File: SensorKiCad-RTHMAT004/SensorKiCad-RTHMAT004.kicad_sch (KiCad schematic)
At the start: 19 parts, among them J1 Conn_02x14_Odd_Even, Q1 SS8050

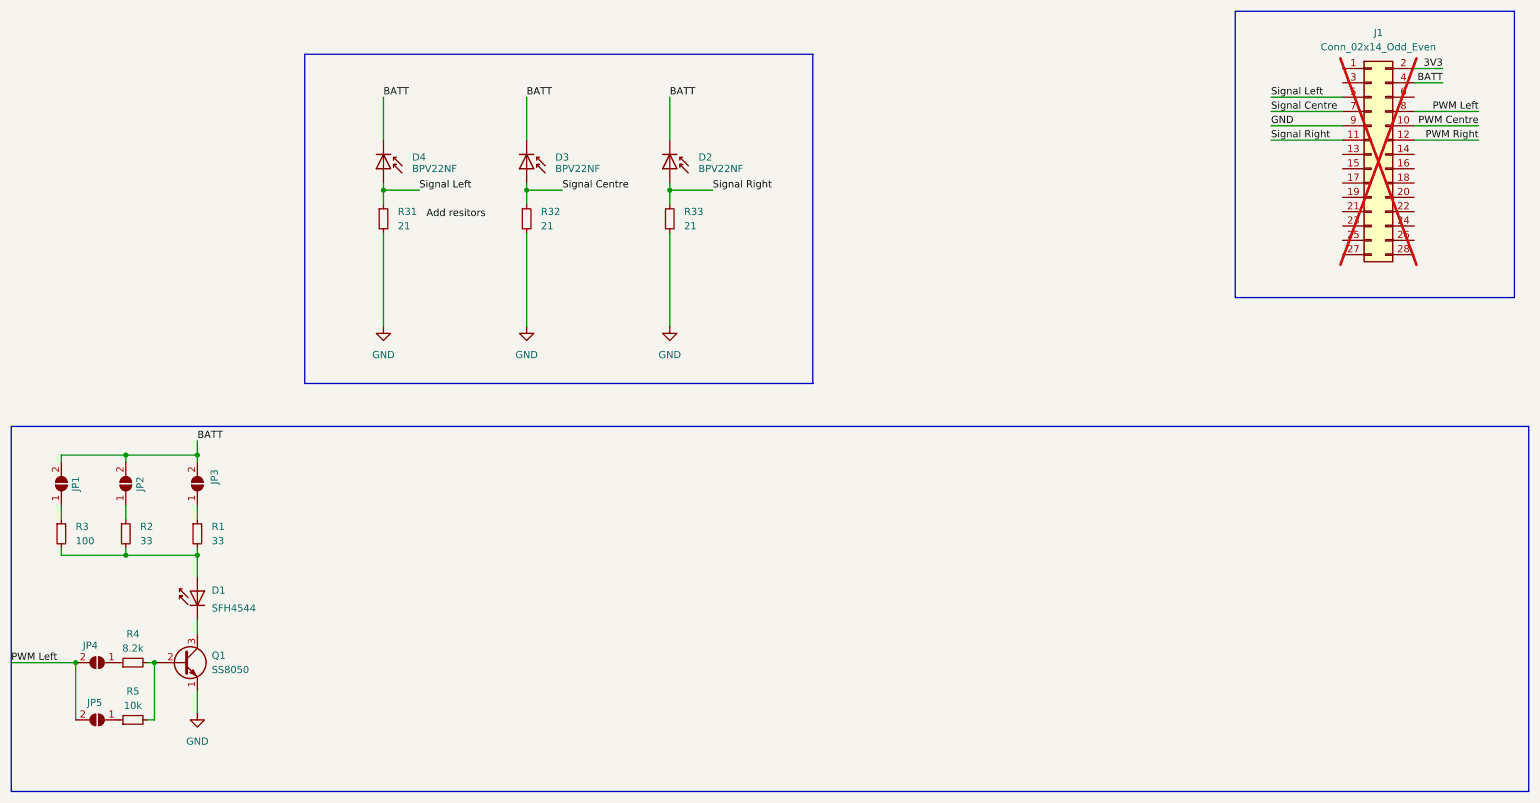
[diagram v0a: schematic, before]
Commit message: Finalising PCB
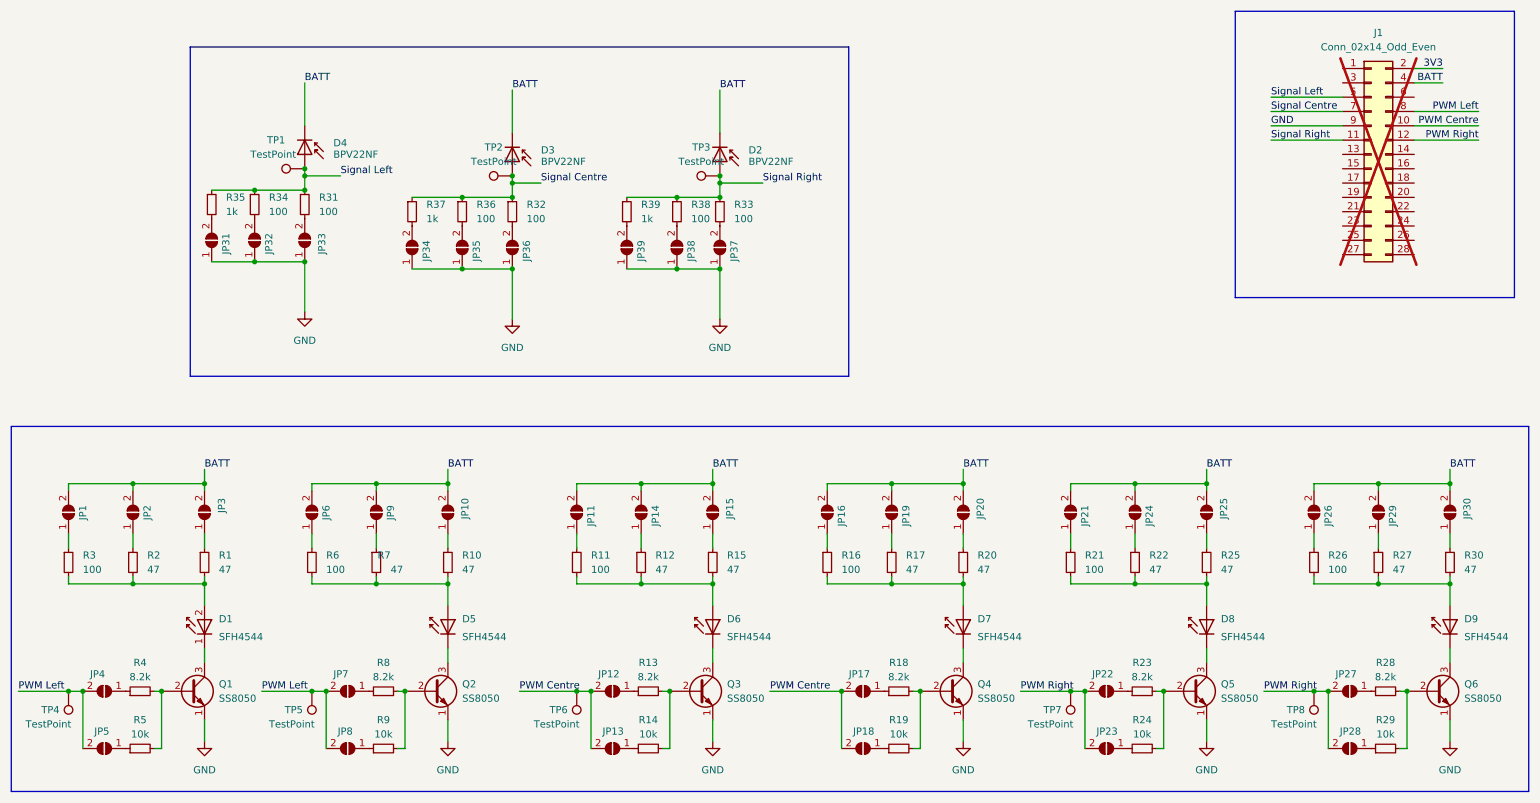
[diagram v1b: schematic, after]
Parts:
- added D5, D6, D7, D8, D9: SFH4544, LED_THT:LED_D5.0mm_Horizontal_O1.27mm_Z3.0mm_IRBlack, symbol LED:SFH4546
- added JP10, JP11, JP12, JP13, JP14, JP15, JP16, JP17, JP18, JP19, JP20, JP21, JP22, JP23, JP24, JP25, JP26, JP27, JP28, JP29, JP30, JP31, JP32, JP33, JP34, JP35, JP36, JP37, JP38, JP39, JP6, JP7, JP8, JP9: SolderJumper_2_Open, Jumper:SolderJumper-2_P1.3mm_Open_Pad1.0x1.5mm, symbol Jumper:SolderJumper_2_Open
- added Q2, Q3, Q4, Q5, Q6: SS8050, Package_TO_SOT_SMD:SOT-23, symbol Transistor_BJT:2N2219
- added R10, R12, R15, R17, R20, R22, R25, R27, R30, R7: 47, Resistor_SMD:R_0805_2012Metric, symbol Device:R_Small
- added R11, R16, R21, R26, R34, R36, R38, R6: 100, Resistor_SMD:R_0805_2012Metric, symbol Device:R_Small
- added R13, R18, R23, R28, R8: 8.2k, Resistor_SMD:R_0805_2012Metric, symbol Device:R_Small
- added R14, R19, R24, R29, R9: 10k, Resistor_SMD:R_1206_3216Metric, symbol Device:R_Small
- added R35, R37, R39: 1k, Resistor_SMD:R_1206_3216Metric, symbol Device:R_Small
- added TP1, TP2, TP3, TP4, TP5, TP6, TP7, TP8: TestPoint, TestPoint:TestPoint_Pad_D2.5mm, symbol Connector:TestPoint
- D1: footprint LED_THT:LED_D3.0mm_IRBlack -> LED_THT:LED_D5.0mm_Horizontal_O1.27mm_Z3.0mm_IRBlack
- D2, D3, D4: LCSC C2900370 -> C130226
- JP1, JP2, JP3, JP4, JP5: footprint (none) -> Jumper:SolderJumper-2_P1.3mm_Open_Pad1.0x1.5mm
- R1, R2: value 33 -> 47; footprint Resistor_SMD:R_0815_2038Metric -> Resistor_SMD:R_0805_2012Metric; LCSC (none) -> C17714
- R3: footprint Resistor_SMD:R_0815_2038Metric -> Resistor_SMD:R_0805_2012Metric; LCSC (none) -> C17901
- R31, R32, R33: value 21 -> 100; footprint Resistor_SMD:R_0815_2038Metric -> Resistor_SMD:R_0805_2012Metric; LCSC (none) -> C17901
- R4: footprint Resistor_SMD:R_0815_2038Metric -> Resistor_SMD:R_0805_2012Metric; LCSC (none) -> C17828
- R5: footprint Resistor_SMD:R_0815_2038Metric -> Resistor_SMD:R_1206_3216Metric; LCSC (none) -> C17902
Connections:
- net BATT: now also JP10.2 (B), JP11.2 (B), JP14.2 (B), JP15.2 (B), JP16.2 (B), JP19.2 (B), JP20.2 (B), JP21.2 (B), JP24.2 (B), JP25.2 (B), JP26.2 (B), JP29.2 (B), JP30.2 (B), JP6.2 (B), JP9.2 (B)
- net GND: now also JP31.1 (A), JP32.1 (A), JP33.1 (A), JP34.1 (A), JP35.1 (A), JP36.1 (A), JP37.1 (A), JP38.1 (A), JP39.1 (A), Q2.1 (E), Q3.1 (E), Q4.1 (E), Q5.1 (E), Q6.1 (E); no longer R31.2, R32.2, R33.2
- net PWM Centre: now also JP12.2 (B), JP13.2 (B), JP17.2 (B), JP18.2 (B), TP6.1
- net PWM Left: now also JP7.2 (B), JP8.2 (B), TP4.1, TP5.1
- net PWM Right: now also JP22.2 (B), JP23.2 (B), JP27.2 (B), JP28.2 (B), TP7.1, TP8.1
- net Signal Centre: now also R36.1, R37.1, TP2.1
- net Signal Left: now also R34.1, R35.1, TP1.1
- net Signal Right: now also R38.1, R39.1, TP3.1
- new net: JP35.2 (B), R36.2
- new net: Q3.2 (B), R13.2, R14.2
- new net: D6.1 (K), Q3.3 (C)
- new net: JP14.1 (A), R12.1
- new net: D6.2 (A), R11.2, R12.2, R15.2
- new net: JP9.1 (A), R7.1
- new net: D5.2 (A), R10.2, R6.2, R7.2
- new net: JP28.1 (A), R29.1
- new net: Q6.2 (B), R28.2, R29.2
- new net: JP12.1 (A), R13.1
- new net: JP32.2 (B), R34.2
- new net: JP26.1 (A), R26.1
- new net: JP37.2 (B), R33.2
- new net: JP31.2 (B), R35.2
- new net: JP23.1 (A), R24.1
- new net: Q5.2 (B), R23.2, R24.2
- new net: JP16.1 (A), R16.1
- new net: JP36.2 (B), R32.2
- new net: JP29.1 (A), R27.1
- new net: D9.2 (A), R26.2, R27.2, R30.2
- new net: JP38.2 (B), R38.2
- new net: JP27.1 (A), R28.1
- new net: JP39.2 (B), R39.2
- new net: JP6.1 (A), R6.1
- new net: JP21.1 (A), R21.1
- new net: JP25.1 (A), R25.1
- new net: JP7.1 (A), R8.1
- new net: JP19.1 (A), R17.1
- new net: D7.2 (A), R16.2, R17.2, R20.2
- new net: JP10.1 (A), R10.1
- new net: D9.1 (K), Q6.3 (C)
- new net: D7.1 (K), Q4.3 (C)
- new net: JP15.1 (A), R15.1
- new net: JP8.1 (A), R9.1
- new net: JP20.1 (A), R20.1
- new net: JP22.1 (A), R23.1
- new net: Q2.2 (B), R8.2, R9.2
- new net: D8.1 (K), Q5.3 (C)
- new net: JP24.1 (A), R22.1
- new net: JP33.2 (B), R31.2
- new net: JP18.1 (A), R19.1
- new net: JP34.2 (B), R37.2
- new net: JP11.1 (A), R11.1
- new net: D8.2 (A), R21.2, R22.2, R25.2
- new net: JP30.1 (A), R30.1
- new net: Q4.2 (B), R18.2, R19.2
- new net: D5.1 (K), Q2.3 (C)
- new net: JP17.1 (A), R18.1
- new net: JP13.1 (A), R14.1
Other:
- moved on the sheet: D2, D3, D4, JP1, JP2, JP3, JP4, JP5, Q1, R1, R2, R3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
